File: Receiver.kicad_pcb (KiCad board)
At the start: 2 copper layers, 30 x 30 mm, 25 parts, among them U1 TL074 (ggf. durch TLV4172IPWR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

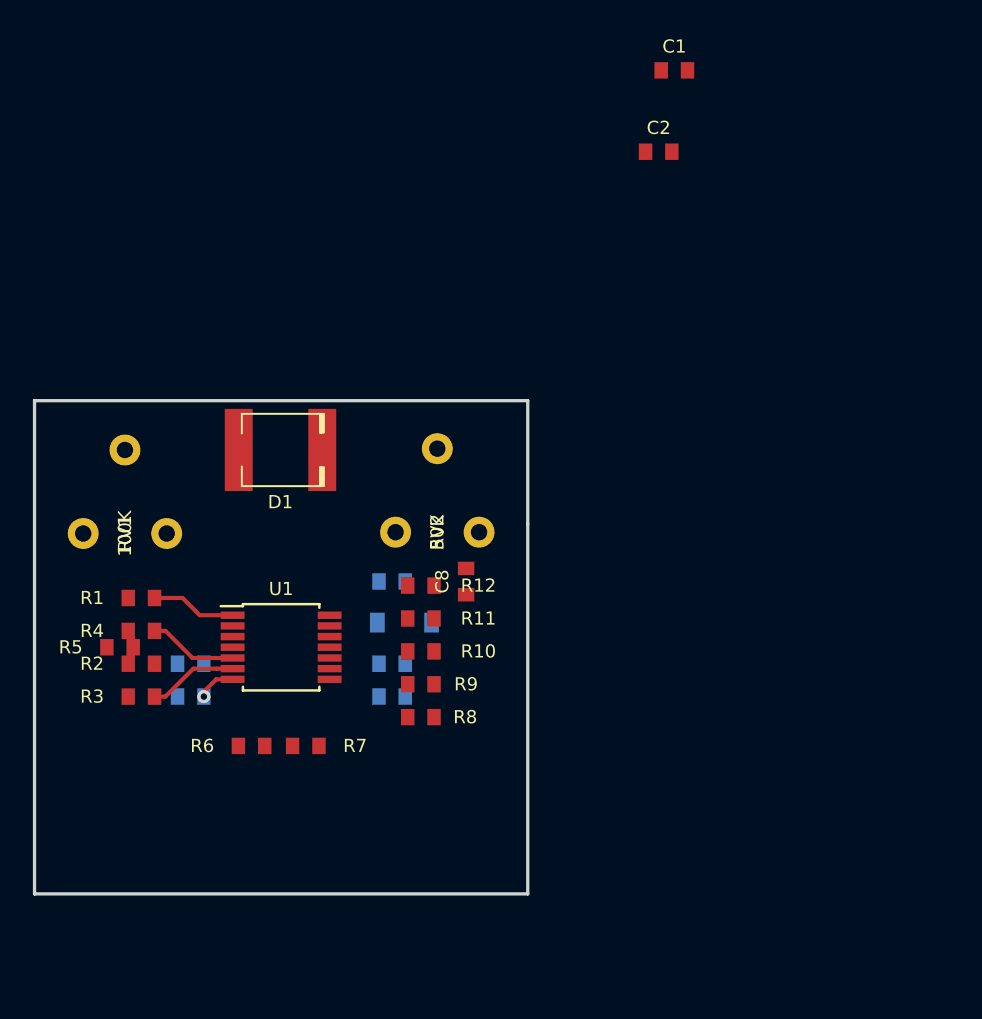
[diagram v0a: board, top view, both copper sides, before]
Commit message: Update schematic and pcb
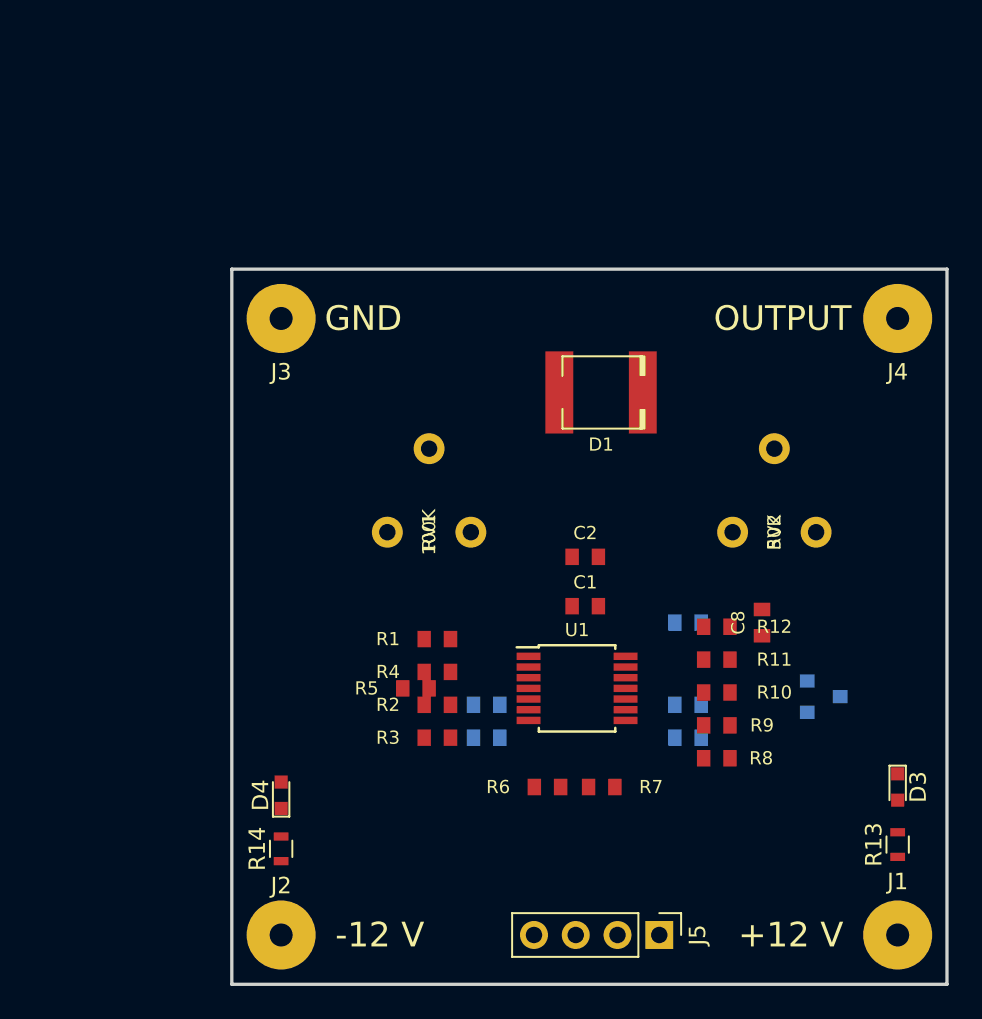
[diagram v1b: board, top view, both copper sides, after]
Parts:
- added D3: LED, LEDs:LED_0603, F.Cu at (127.5, 118.5)
- added D4: LED, LEDs:LED_0603, F.Cu at (90.0, 119.0)
- added J1: +12V, optoreceiver:Hirschmann_MST201, F.Cu at (127.5, 127.5)
- added J2: -12V, optoreceiver:Hirschmann_MST201, F.Cu at (90.0, 127.5)
- added J3: GND, optoreceiver:Hirschmann_MST201, F.Cu at (90.0, 90.0)
- added J4: OUTPUT, optoreceiver:Hirschmann_MST201, F.Cu at (127.5, 90.0)
- added J5: Conn_01x04, Pin_Headers:Pin_Header_Straight_1x04_Pitch2.54mm, F.Cu at (113.0, 127.5)
- added R13: 1k, Resistors_SMD:R_0603, F.Cu at (127.5, 122.0)
- added R14: 1k, Resistors_SMD:R_0603, F.Cu at (90.0, 122.3)
- D2: value Schottky -> BAT54; footprint Diode_SMD:D_SOD-123 -> Diodes_SMD:D_SOT-23_ANK
- moved C1 33.0 mm to (108.5, 107.5)
- moved D2 25.9 mm to (123.0, 113.0)
- moved C2 25.0 mm to (108.5, 104.5)
- moved RV2 20.5 mm to (120.0, 103.0)
- moved D1 19.8 mm to (112.0, 94.5)
- moved RV1 18.5 mm to (99.0, 103.0)
- moved C3 18.2 mm to (102.5, 115.5)
- moved C4 18.2 mm to (102.5, 113.5)
- moved C5 18.2 mm to (114.8, 113.5)
- moved C6 18.2 mm to (114.8, 115.5)
- moved C7 18.2 mm to (114.8, 108.5)
- moved C8 18.2 mm to (119.2, 108.5)
- moved R1 18.2 mm to (99.5, 109.5)
- moved R10 18.2 mm to (116.5, 112.8)
- moved R11 18.2 mm to (116.5, 110.8)
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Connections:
- net Net-(C8-Pad2) renamed /OUTPUT
- U1 pad 4: Net-(U1-Pad4) -> +12V
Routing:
- net Net-(C4-Pad1): track 5.45 -> 0.00 mm
- net Net-(R4-Pad1): track 5.43 -> 0.00 mm
- net Net-(R1-Pad2): track 5.18 -> 0.00 mm
- net Net-(C3-Pad1): track 2.36 -> 0.00 mm, vias 1 -> 0
- added copper zone on B.Cu, net GND
- added copper zone on F.Cu, net GND
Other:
- board size 30 x 30 mm -> 43.5 x 43.5 mm
- board text added: "+12 V"
- board text added: "-12 V"
- board text added: "GND"
- board text added: "OUTPUT"

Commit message: Add files via upload
- Platzierung und Silkscreen angepasst
- 3D Modelle ergänzt
- aktuelle Renderbilder erzeugt
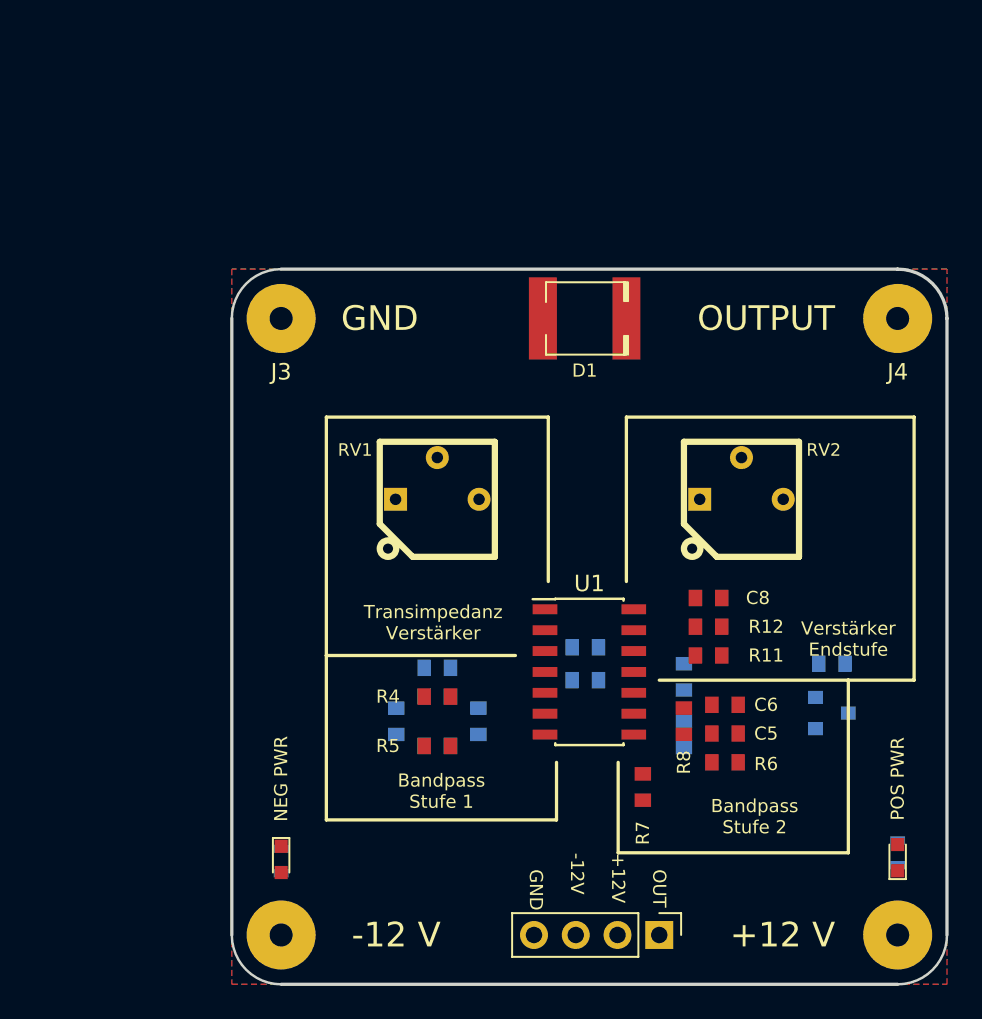
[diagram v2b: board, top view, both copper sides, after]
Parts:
- C1, C2, R1, R10, R13, R14, R2, R3, R9: moved to B.Cu
- C5, C6: moved to F.Cu
- D1: footprint kicadlibs:Osram_DIL2_4.3x4.65mm_P5.08mm -> OptoDevice:Osram_SMD2_4.3x4.65mm_P5.08mm
- RV1, RV2: footprint SparkFun-Electromechanical:TRIM_POT -> User-Submitted:BOURNS-3362P_pot
- U1: footprint Package_SO:TSSOP-14_4.4x5mm_P0.65mm -> Package_SO:SOIC-14_3.9x8.7mm_P1.27mm
- moved R6 10.9 mm to (117.0, 117.0)
- moved C7 9.10 mm to (123.5, 111.0), turned to 0 degrees
- moved C2 7.50 mm to (108.5, 112.0)
- moved D1 4.61 mm to (111.0, 90.0)
- moved D3 4.30 mm to (127.5, 122.8), turned to 90 degrees
- moved D4 3.90 mm to (90.0, 122.9), turned to 270 degrees
- moved R5 3.73 mm to (99.5, 116.0)
- moved C8 3.58 mm to (116.0, 107.0), turned to 0 degrees
- moved C3 3.04 mm to (99.5, 116.0)
- moved C4 3.04 mm to (99.5, 113.0)
- moved C6 3.01 mm to (117.0, 113.5), turned to 0 degrees
- moved R8 3.01 mm to (114.5, 114.5), turned to 270 degrees
- moved C5 2.85 mm to (117.0, 115.2), turned to 0 degrees
- moved RV2 2.83 mm to (118.0, 101.0), turned to 0 degrees
- moved R2 2.69 mm to (97.0, 114.5), turned to 270 degrees
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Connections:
- U1 pad 11: Net-(U1-Pad11) -> -12V
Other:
- outline, holes or cut-outs redrawn
- board text added: "+12V"
- board text added: "-12V"
- board text added: "Bandpass Stufe 1"
- board text added: "Bandpass Stufe 2"
- board text added: "Gleichrichter"
- board text added: "NEG PWR"
- board text added: "OUT"
- board text added: "OptoReceiver V0.1"
- board text added: "POS PWR"
- board text added: "Transimpedanz Verstärker"
- board text added: "Verstärker Endstufe"
